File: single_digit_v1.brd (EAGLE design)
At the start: 101.6 x 50.8 mm, 85 parts

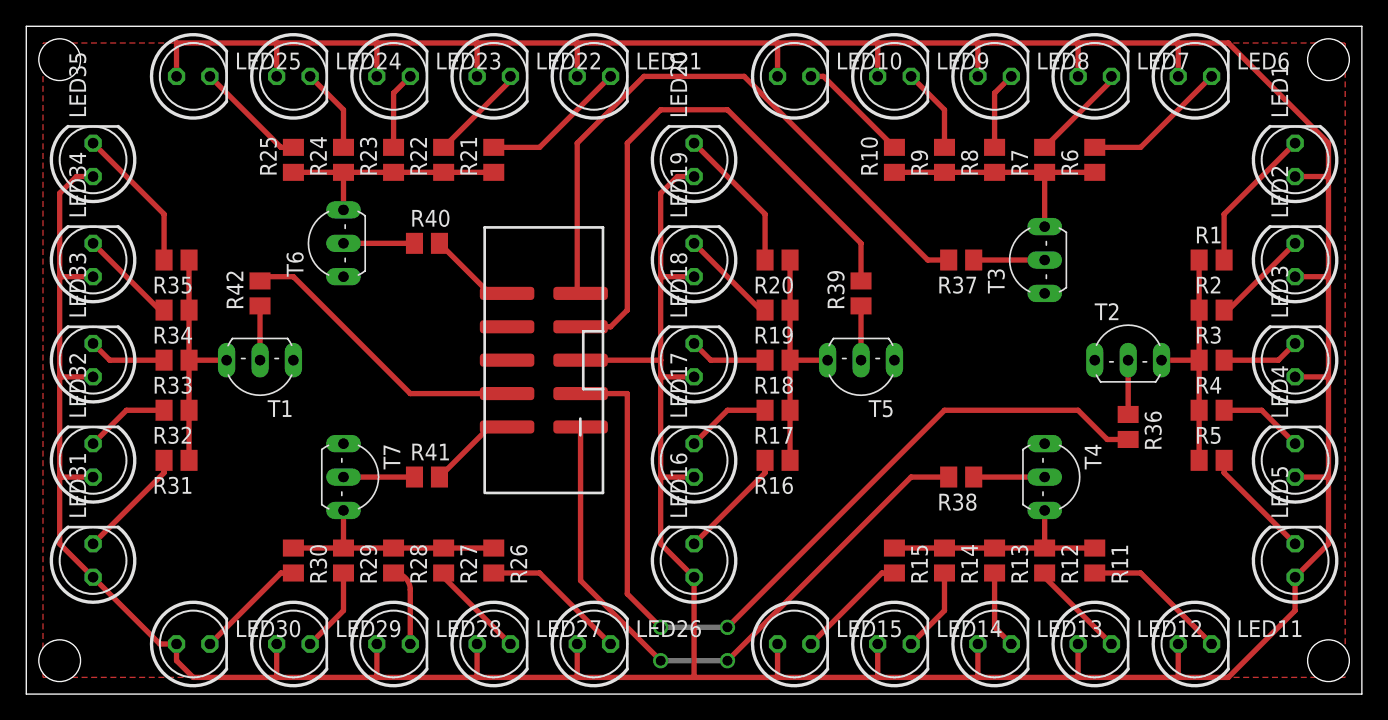
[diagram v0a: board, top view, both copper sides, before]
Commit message: ready for production
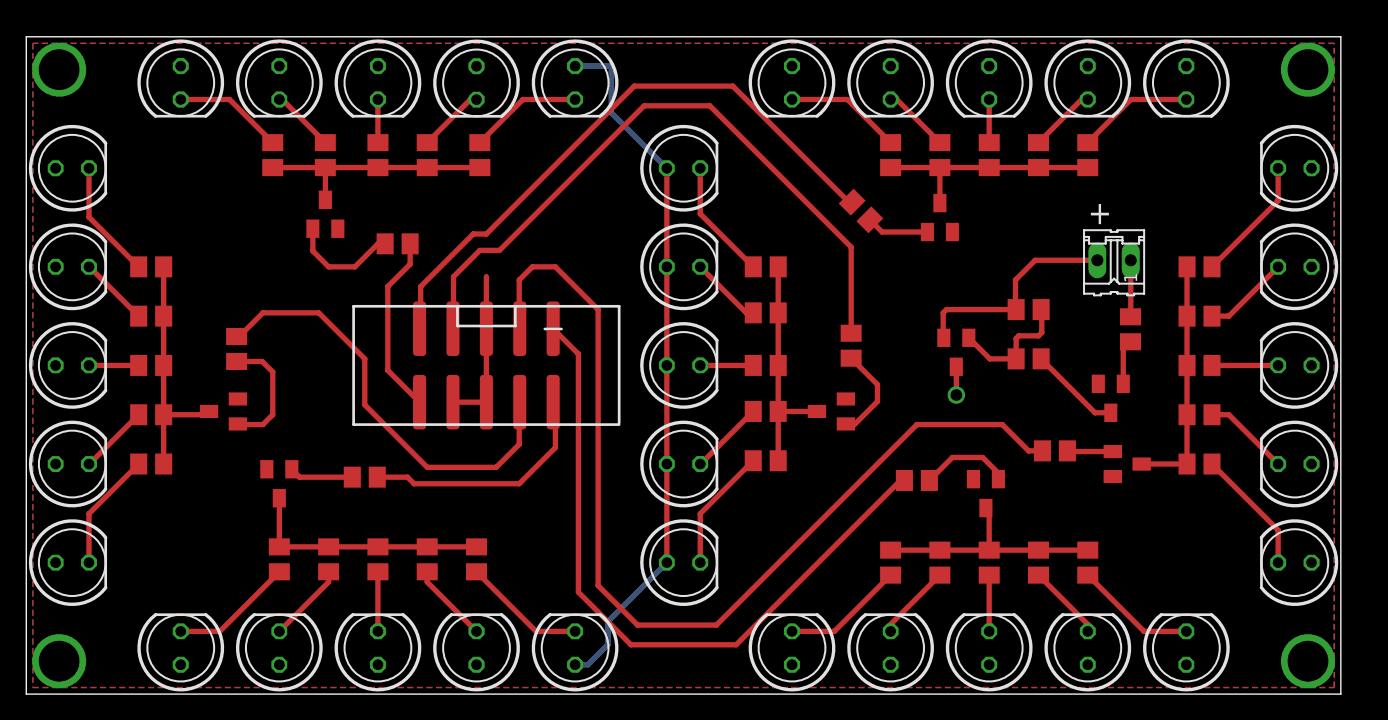
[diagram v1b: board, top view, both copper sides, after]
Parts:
- added R43, R44, R45: (no value), rcl:M0805
- added SL1: (no value), con-amp-quick:02P
- added T8, T9: (no value), transistor:SOT23-BEC
- T1, T2, T3, T4, T5, T6, T7: device transistor-neu-to92:TO92-EBC -> transistor:SOT23-BEC
- moved T2 9.17 mm to (83.8, 17.5), turned to 270 degrees
- moved R37 8.48 mm to (63.5, 36.8), turned to 135 degrees
- moved T3 7.44 mm to (69.5, 36.2), turned to 0 degrees
- moved T7 6.17 mm to (19.2, 16.0), turned to 180 degrees
- moved T4 5.88 mm to (73.0, 15.2), turned to 180 degrees
- moved R36 5.86 mm to (78.2, 18.5), turned to 180 degrees
- moved R41 4.73 mm to (25.8, 16.5)
- moved R42 4.59 mm to (16.0, 26.2)
- moved JP1 4.39 mm to (35.0, 25.0), turned to 270 degrees
- moved R39 4.05 mm to (62.8, 26.5)
- moved T1 3.83 mm to (15.0, 21.5), turned to 90 degrees
- moved T5 3.46 mm to (61.2, 21.5), turned to 90 degrees
- moved R38 3.38 mm to (67.8, 16.2)
- moved R40 2.23 mm to (28.2, 34.2)
- moved T6 2.21 mm to (22.8, 36.5), turned to 0 degrees
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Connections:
- new net N$50: R43.2, T8.C
- new net N$51: R43.1, R44.2, T9.B
- new net N$52: R45.1, T8.B
- new net N$53: R45.2, SL1.1
- new net VCC: LED1.A, LED10.A, LED11.A, LED12.A, LED13.A, LED14.A, LED15.A, LED16.A, LED17.A, LED18.A, LED19.A, LED2.A, LED20.A, LED21.A, LED22.A, LED23.A, LED24.A, LED25.A, LED26.A, LED27.A, LED28.A, LED29.A, LED3.A, LED30.A, LED31.A, LED32.A, LED33.A, LED34.A, LED35.A, LED4.A, LED5.A, LED6.A, LED7.A, LED8.A, LED9.A, T9.C
- net +5V: now also R44.1, SL1.2, T9.E; no longer JP1.5, LED1.A, LED10.A, LED11.A, LED12.A, LED13.A, LED14.A, LED15.A, LED16.A, LED17.A, LED18.A, LED19.A, LED2.A, LED20.A, LED21.A, LED22.A, LED23.A, LED24.A, LED25.A, LED26.A, LED27.A, LED28.A, LED29.A, LED3.A, LED30.A, LED31.A, LED32.A, LED33.A, LED34.A, LED35.A, LED4.A, LED5.A, LED6.A, LED7.A, LED8.A, LED9.A
- net GNDA: now also JP1.5, JP1.8, T8.E
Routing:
- net +5V: track 378.9 -> 16.7 mm
- net VCC: track 0.00 -> 55.7 mm, vias 0 -> 1
- net GNDA: track 0.00 -> 12.1 mm
- net S6: track 6.72 -> 18.4 mm
- net S7: track 22.6 -> 33.1 mm
- net N$51: track 0.00 -> 9.72 mm
- net S1: track 65.7 -> 74.7 mm, vias 2 -> 0
- net S5: track 6.72 -> 13.8 mm
- net N$50: track 0.00 -> 7.00 mm
- net S4: track 43.7 -> 50.6 mm
- net N$49: track 4.13 -> 9.31 mm
- net S3: track 48.0 -> 52.5 mm, vias 2 -> 0
- net N$53: track 0.00 -> 4.31 mm
- net N$52: track 0.00 -> 3.43 mm
- net N$42: track 4.13 -> 7.23 mm
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- added copper zone on layer 16, net VCC
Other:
- board size 101.6 x 50.8 mm -> 100 x 50 mm
- board text added: "+"
